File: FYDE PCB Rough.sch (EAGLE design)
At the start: 4 parts, among them P1 SEN-11574, U1 MCU-MCP3008-I/P(DIP16-7.62MM), X1 RASPI_BOARD_B+_HDC

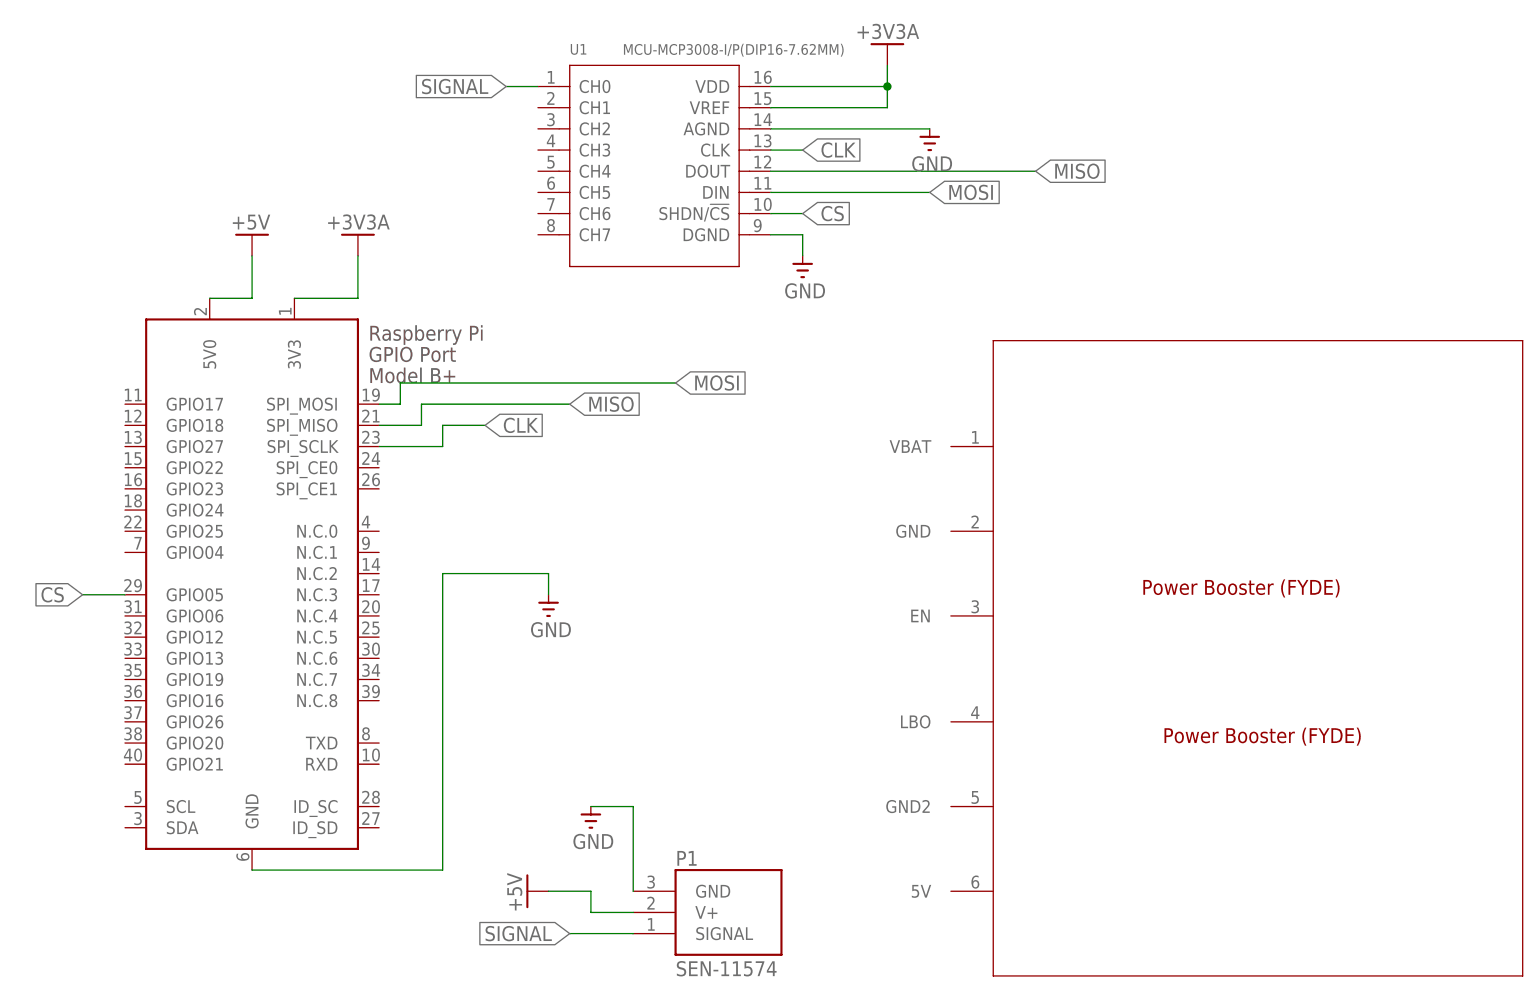
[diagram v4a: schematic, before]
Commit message: Add files via upload
new powerbooster (with library)
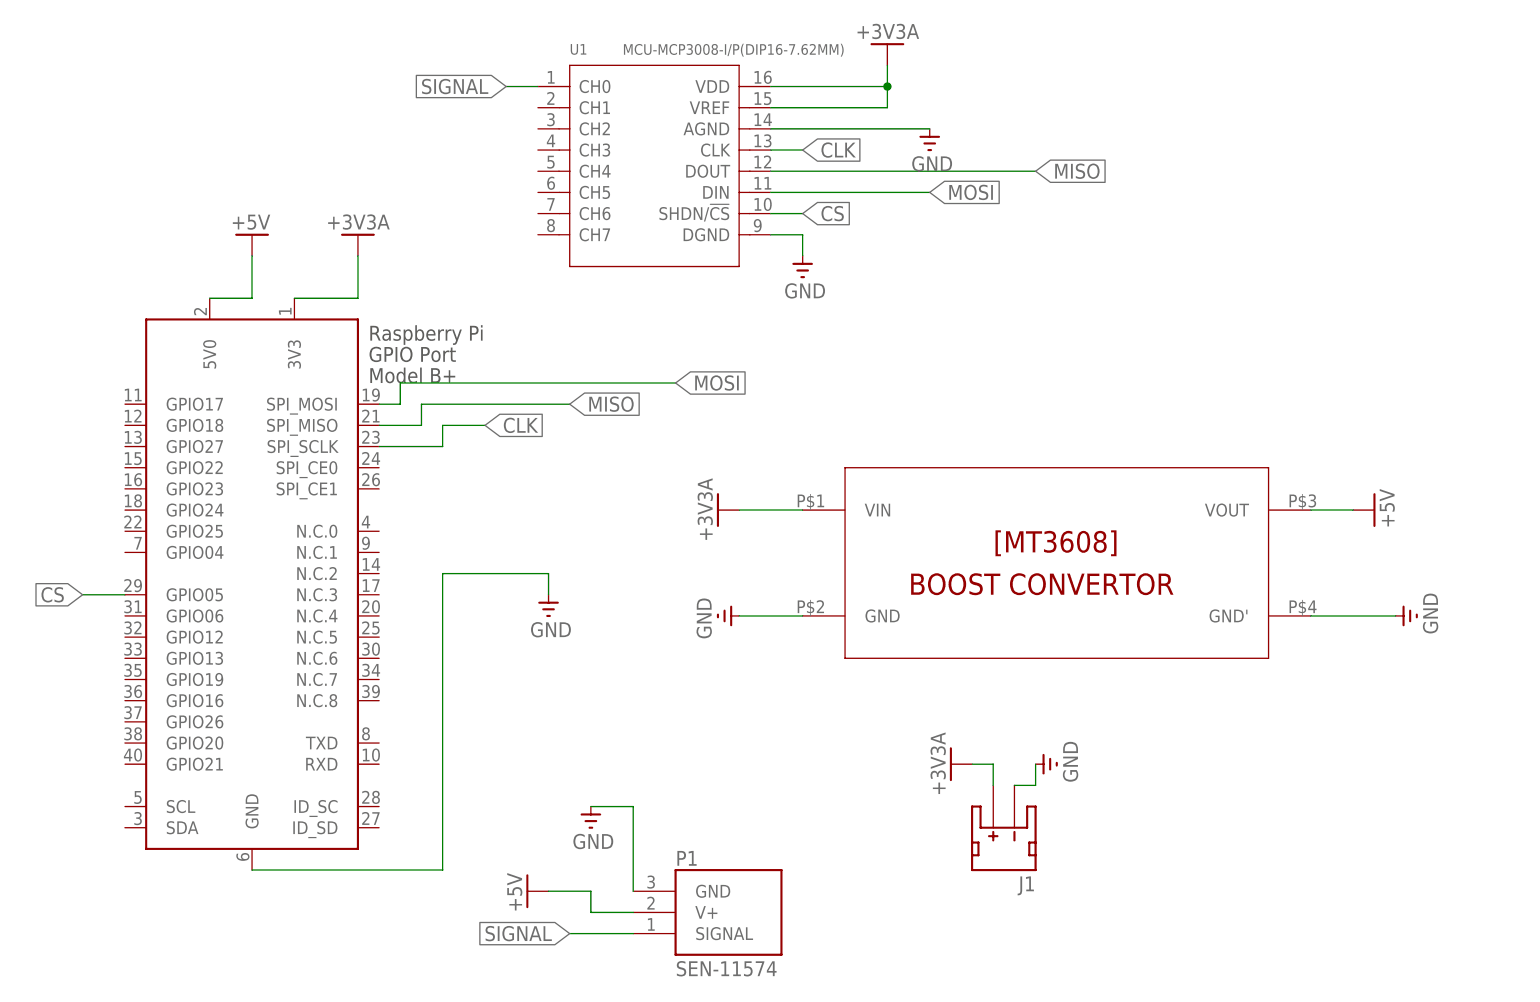
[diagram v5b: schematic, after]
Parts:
- removed U$1: ADAFRUITPOWERBOOSTER(FYDE), Adafruit-PowerBoost-FYDE:ADAFRUITPOWERBOOSTER(FYDE)
- added J1: (no value), SparkFun-Connectors:JST_2MM_MALE
- added U$2: MT3608, MT3608:MT3608
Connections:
- net +3V3A: now also J1.+, U$2.VIN
- net +5V: now also U$2.VOUT
- net GND: now also J1.-, U$2.GND, U$2.GND'
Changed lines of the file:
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@@
 <layer number="112" name="tSilk" color="7" fill="1" visible="no" active="yes"/>
 <layer number="113" name="ReferenceLS" color="7" fill="1" visible="no" active="no"/>
+<layer number="114" name="Badge_Outline" color="7" fill="1" visible="yes" active="yes"/>
+<layer number="115" name="ReferenceISLANDS" color="7" fill="1" visible="yes" active="yes"/>
 <layer number="116" name="Patch_BOT" color="9" fill="4" visible="no" active="yes"/>
 <layer number="118" name="Rect_Pads" color="7" fill="1" visible="no" active="no"/>
@@
 <parts>
 <part name="P1" library="SEN-11574" deviceset="SEN-11574" device=""/>
-<part name="U$1" library="Adafruit-PowerBoost-FYDE" deviceset="ADAFRUITPOWERBOOSTER(FYDE)" device=""/>
 <part name="U1" library="MCU-MCP3008-I_P_DIP16-7.62MM_" deviceset="MCU-MCP3008-I/P(DIP16-7.62MM)" device=""/>
 <part name="GND1" library="supply" deviceset="GND" device=""/>
@@
 <part name="V4" library="supply0" deviceset="+5V" device=""/>
 <part name="X1" library="raspberrypi_bastelstube_v13" deviceset="RASPI_BOARD_B+" device="_HDC"/>
+<part name="U$2" library="MT3608" deviceset="MT3608" device=""/>
+<part name="GND6" library="supply" deviceset="GND" device=""/>
+<part name="GND5" library="supply" deviceset="GND" device=""/>
+<part name="V5" library="supply0" deviceset="+5V" device=""/>
+<part name="V6" library="supply0" deviceset="+3V3A" device=""/>
+<part name="J1" library="SparkFun-Connectors" library_urn="urn:adsk.eagle:library:513" deviceset="JST_2MM_MALE" device="" package3d_urn="urn:adsk.eagle:package:38042/1"/>
+<part name="V7" library="supply0" deviceset="+3V3A" device=""/>
+<part name="GND7" library="supply" deviceset="GND" device=""/>
 </parts>
 <sheets>
@@
 <instances>
 <instance part="P1" gate="G$1" x="-99.06" y="96.52"/>
-<instance part="U$1" gate="G$1" x="-50.8" y="88.9"/>
 <instance part="U1" gate="G$1" x="-101.6" y="185.42"/>
 <instance part="GND1" gate="1" x="-114.3" y="132.08"/>
@@
 <instance part="V4" gate="1" x="-149.86" y="177.8"/>
 <instance part="X1" gate="G$1" x="-149.86" y="142.24"/>
+<instance part="U$2" gate="G$1" x="-78.74" y="127"/>
+<instance part="GND6" gate="1" x="-93.98" y="132.08" rot="R270"/>
+<instance part="GND5" gate="1" x="-10.16" y="132.08" rot="R90"/>
+<instance part="V5" gate="1" x="-15.24" y="144.78" rot="R270"/>
+<instance part="V6" gate="G$1" x="-93.98" y="144.78" rot="R90"/>
+<instance part="J1" gate="G$1" x="-58.42" y="106.68" rot="R180"/>
+<instance part="V7" gate="G$1" x="-66.04" y="114.3" rot="R90"/>
+<instance part="GND7" gate="1" x="-53.34" y="114.3" rot="R90"/>
 </instances>
 <busses>
@@
 <wire x1="-109.22" y1="109.22" x2="-104.14" y2="109.22" width="0.1524" layer="91"/>
 <wire x1="-104.14" y1="109.22" x2="-104.14" y2="99.06" width="0.1524" layer="91"/>
+</segment>
+<segment>
+<pinref part="GND6" gate="1" pin="GND"/>
+<pinref part="U$2" gate="G$1" pin="GND"/>
+<wire x1="-91.44" y1="132.08" x2="-83.82" y2="132.08" width="0.1524" layer="91"/>
+</segment>
+<segment>
+<pinref part="GND5" gate="1" pin="GND"/>
+<pinref part="U$2" gate="G$1" pin="GND'"/>
+<wire x1="-12.7" y1="132.08" x2="-22.86" y2="132.08" width="0.1524" layer="91"/>
+</segment>
+<segment>
+<pinref part="GND7" gate="1" pin="GND"/>
+<pinref part="J1" gate="G$1" pin="-"/>
+<wire x1="-55.88" y1="114.3" x2="-55.88" y2="111.76" width="0.1524" layer="91"/>
+<wire x1="-55.88" y1="111.76" x2="-58.42" y2="111.76" width="0.1524" layer="91"/>
 </segment>
 </net>
@@
 <junction x="-73.66" y="195.58"/>
 </segment>
+<segment>
+<pinref part="U$2" gate="G$1" pin="VIN"/>
+<pinref part="V6" gate="G$1" pin="+3V3A"/>
+<wire x1="-83.82" y1="144.78" x2="-91.44" y2="144.78" width="0.1524" layer="91"/>
+</segment>
+<segment>
+<pinref part="V7" gate="G$1" pin="+3V3A"/>
+<pinref part="J1" gate="G$1" pin="+"/>
+<wire x1="-63.5" y1="114.3" x2="-60.96" y2="114.3" width="0.1524" layer="91"/>
+<wire x1="-60.96" y1="114.3" x2="-60.96" y2="111.76" width="0.1524" layer="91"/>
+</segment>
 </net>
 <net name="CLK" class="0">
@@
 <wire x1="-149.86" y1="170.18" x2="-154.94" y2="170.18" width="0.1524" layer="91"/>
 </segment>
+<segment>
+<pinref part="V5" gate="1" pin="+5V"/>
+<pinref part="U$2" gate="G$1" pin="VOUT"/>
+<wire x1="-17.78" y1="144.78" x2="-22.86" y2="144.78" width="0.1524" layer="91"/>
+</segment>
 </net>
 <net name="CS" class="0">
@@
 </sheet>
 </sheets>
+<errors>
+</errors>
 </schematic>
 </drawing>
+<compatibility>
+<note version="8.2" severity="warning">
+Since Version 8.2, EAGLE supports online libraries. The ids
+of those online libraries will not be understood (or retained)
+with this version.
+</note>
+<note version="8.3" severity="warning">
+Since Version 8.3, EAGLE supports URNs for individual library
+assets (packages, symbols, and devices). The URNs of those assets
+will not be understood (or retained) with this version.
+</note>
+<note version="8.3" severity="warning">
+Since Version 8.3, EAGLE supports the association of 3D packages
+with devices in libraries, schematics, and board files. Those 3D
+packages will not be understood (or retained) with this version.
+</note>
+</compatibility>
 </eagle>
